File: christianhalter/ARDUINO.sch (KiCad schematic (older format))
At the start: 0 parts

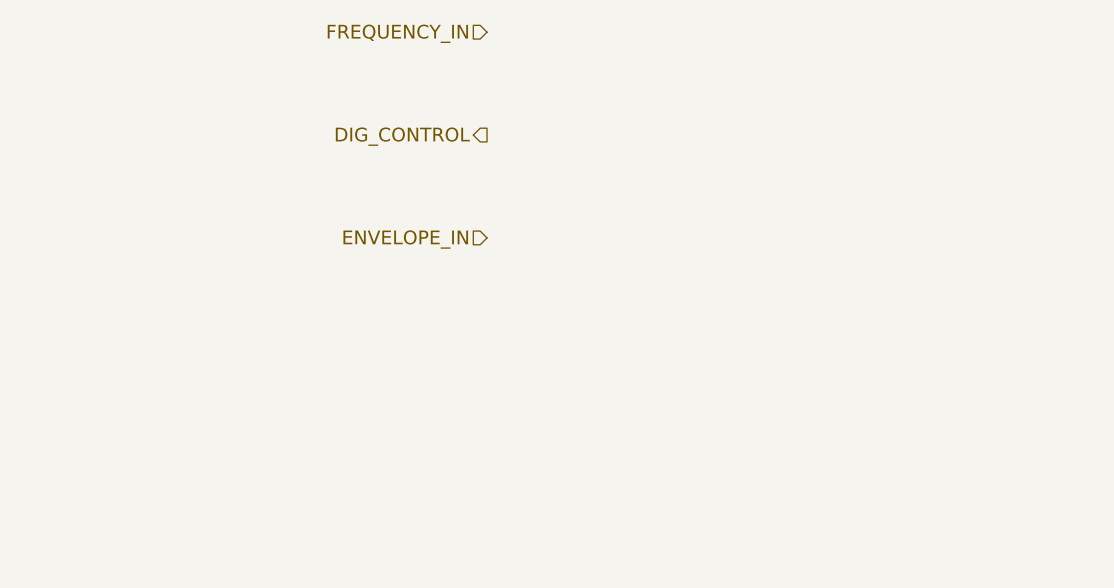
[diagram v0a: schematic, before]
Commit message: componente nuevo
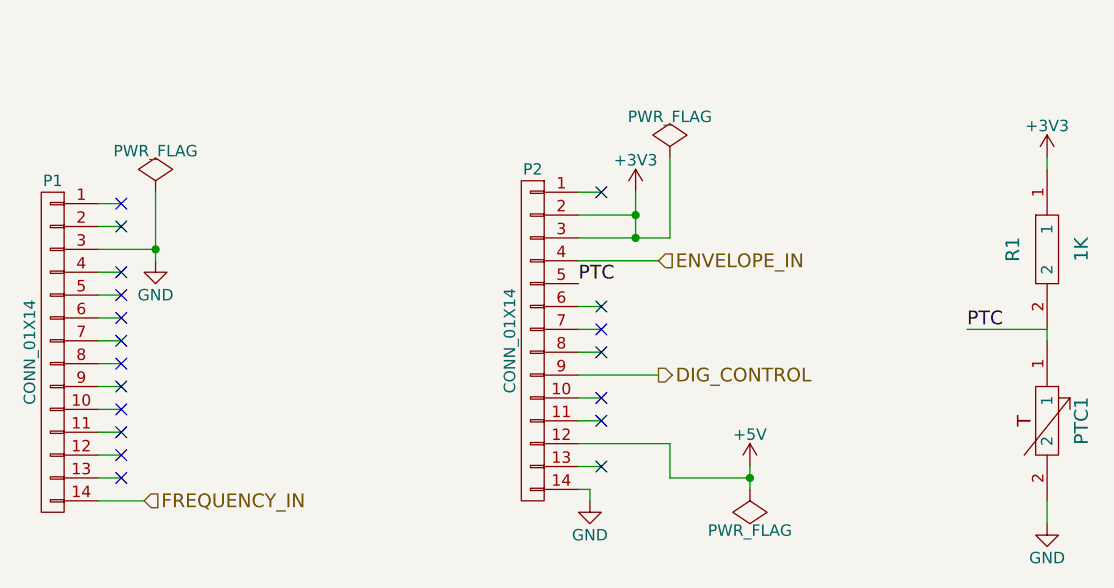
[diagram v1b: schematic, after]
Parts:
- added P1, P2: CONN_01X14, halter:PINHEAD1-14, symbol CONN_01X14
- added PTC1: PTC_HandSoldering, halter:R_0805_HandSoldering, symbol PTC_HandSoldering
- added R1: 1K, halter:R_0805_HandSoldering, symbol Resistor_0805_HandSoldering
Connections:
- net DIG_CONTROL: now also P2.9 (P9)
- net ENVELOPE_IN: now also P2.4 (P4)
- net FREQUENCY_IN: now also P1.14 (P14)
- new net +3V3: P2.2 (P2), P2.3 (P3), R1.1
- new net +5V: P2.12 (P12)
- new net GND: P1.3 (P3), P2.14 (P14), PTC1.2
- new net PTC: P2.5 (P5), PTC1.1, R1.2
- no-connect marks 0 -> 19
